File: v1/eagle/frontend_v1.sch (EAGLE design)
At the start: 57 parts, among them IC1 TINY24/44/84-SSU, IC2 AD5339MSOP8, IC3 LM4041A12DCK, Q10 TIP42C, Q9 TIP41C, T3 TIP35CVERTICAL, T4 TIP35CVERTICAL, U2 LM35DT, U3 LM35DT

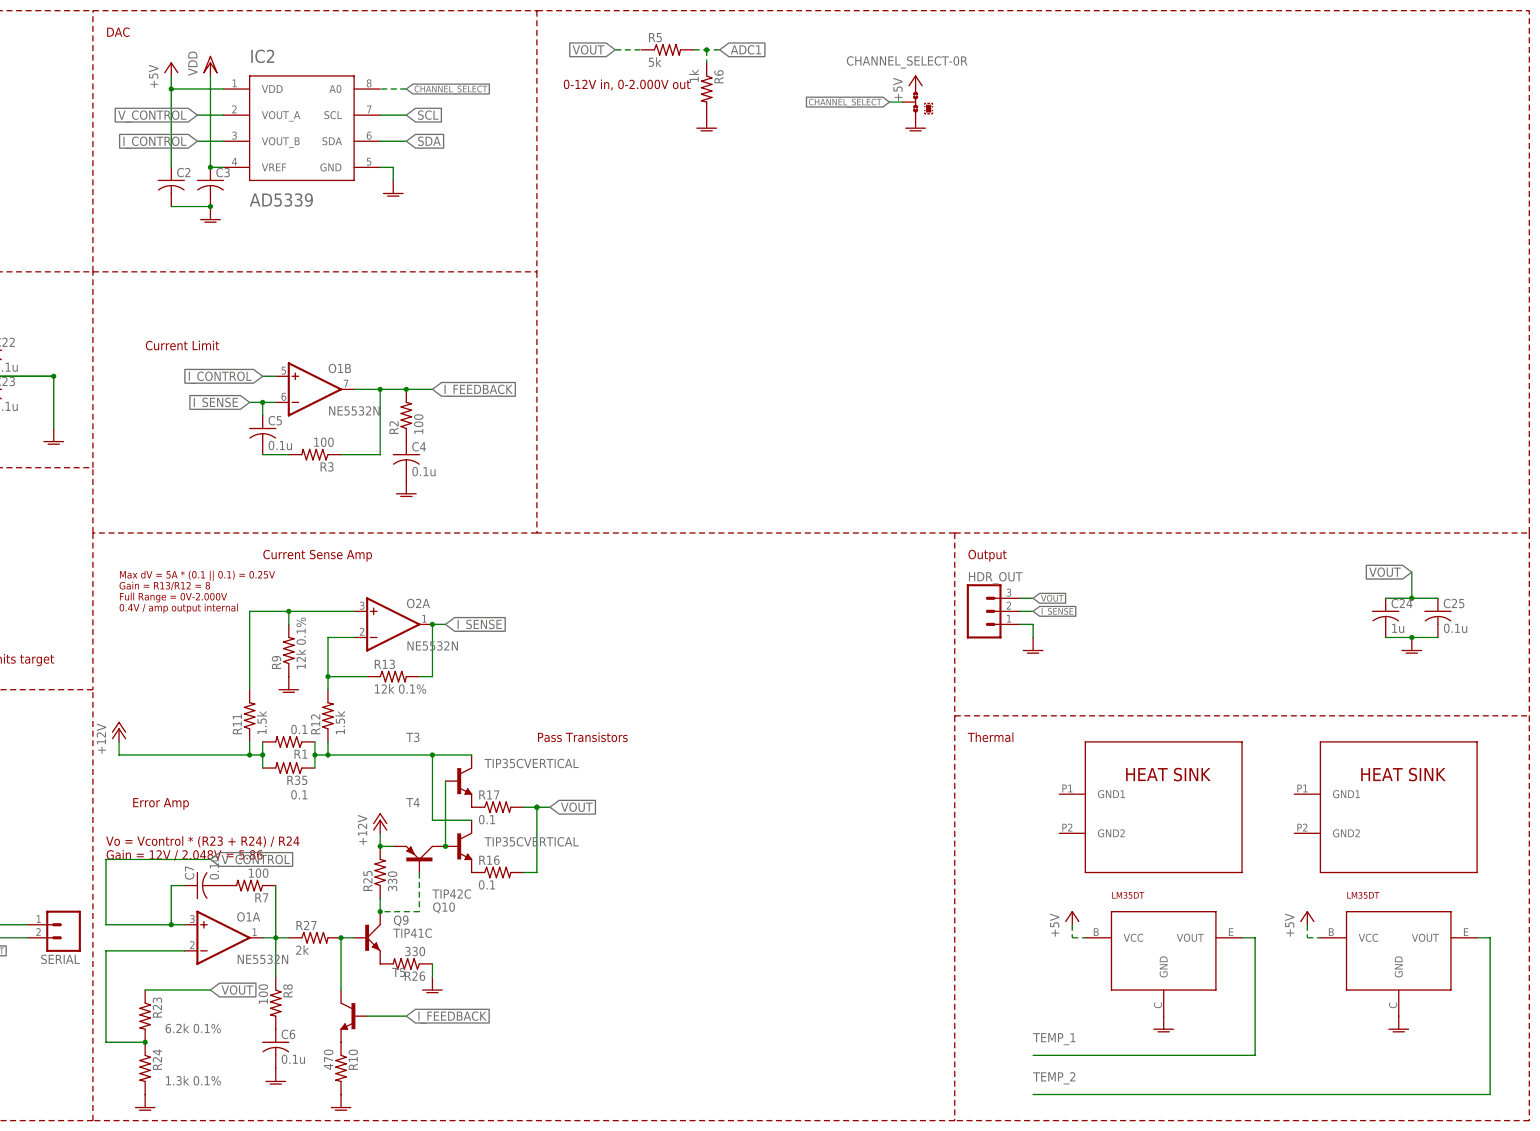
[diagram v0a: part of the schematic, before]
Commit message: minor changes
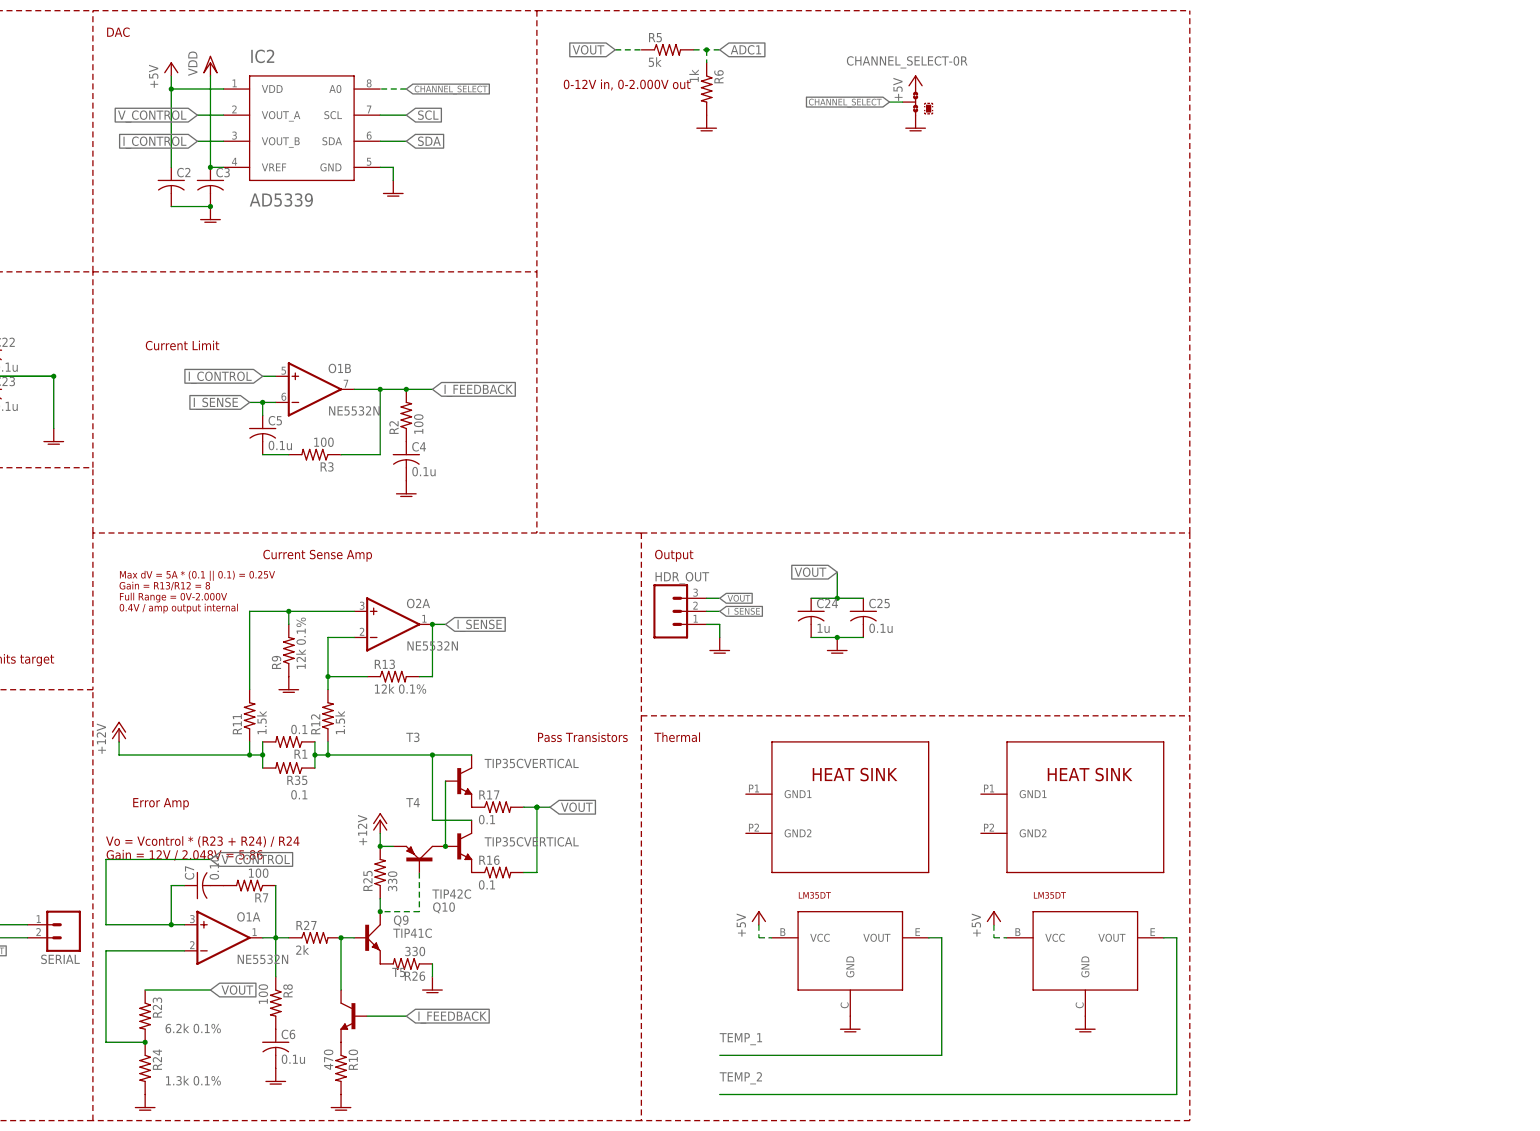
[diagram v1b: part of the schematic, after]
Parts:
- R1, R16, R17, R35: device rcl:R-US_R2010 -> rcl:R-US_R2512
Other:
- moved on the sheet: C24, C25, HDR_OUT
